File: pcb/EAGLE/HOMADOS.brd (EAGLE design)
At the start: 128.3 x 67.3 mm, 78 parts, among them P1 39-30-02?, P10 39-30-02?, P11 39-30-02?, P12 39-30-02?, P13 39-30-02?, P14 39-30-02?, P15 39-30-02?, P16 39-30-02?, P17 39-30-02?, P18 39-30-02?, P2 39-30-02?, P3 39-30-02?, P4 39-30-02?, P5 39-30-02?, P6 39-30-02?, P7 39-30-02?, P8 39-30-02?, P9 39-30-02?, Q1 T460, Q10 T460, Q11 T460, Q12 T460, Q13 T460, Q14 T460, Q15 T460, Q16 T460, Q2 T460, Q3 T460, Q4 T460, Q5 T460, Q6 T460, Q7 T460, Q8 T460, Q9 T460, U2 ARDUINO-MEGAPRO-5V

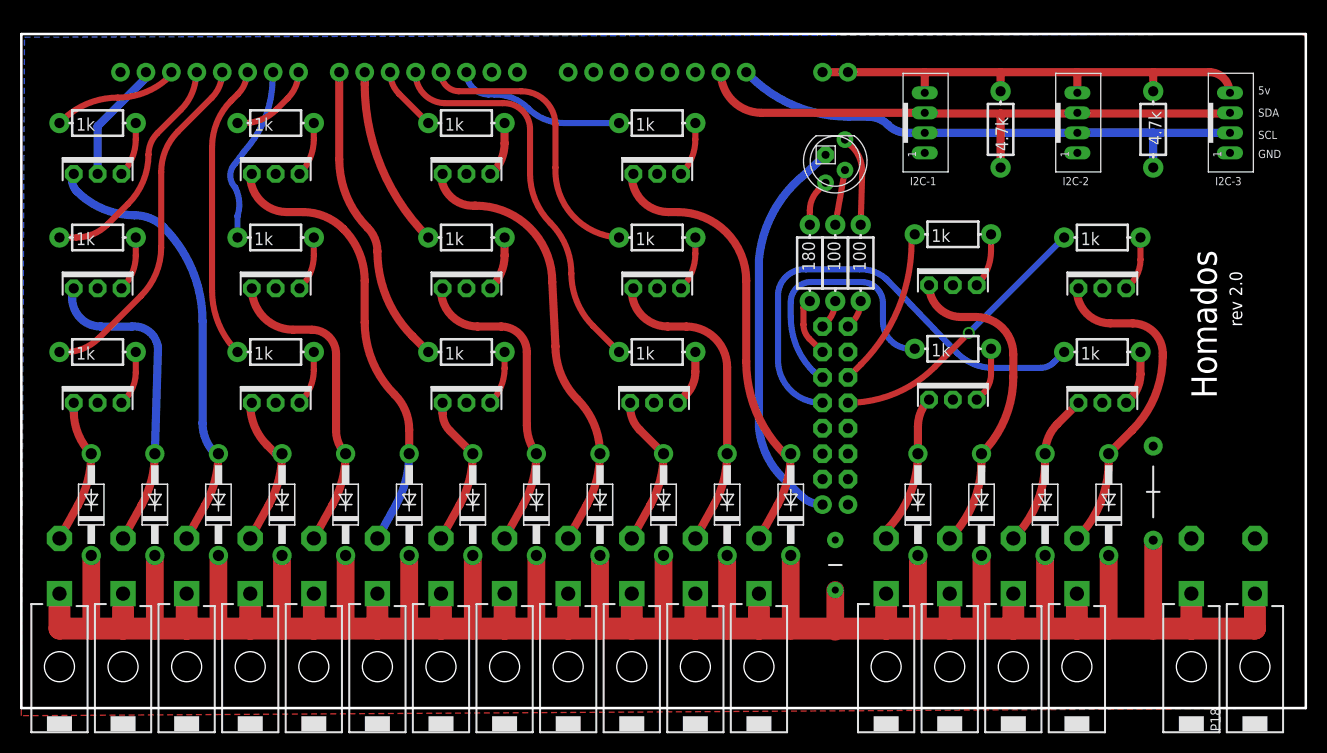
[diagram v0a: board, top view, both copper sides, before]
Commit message: finished revision of homados
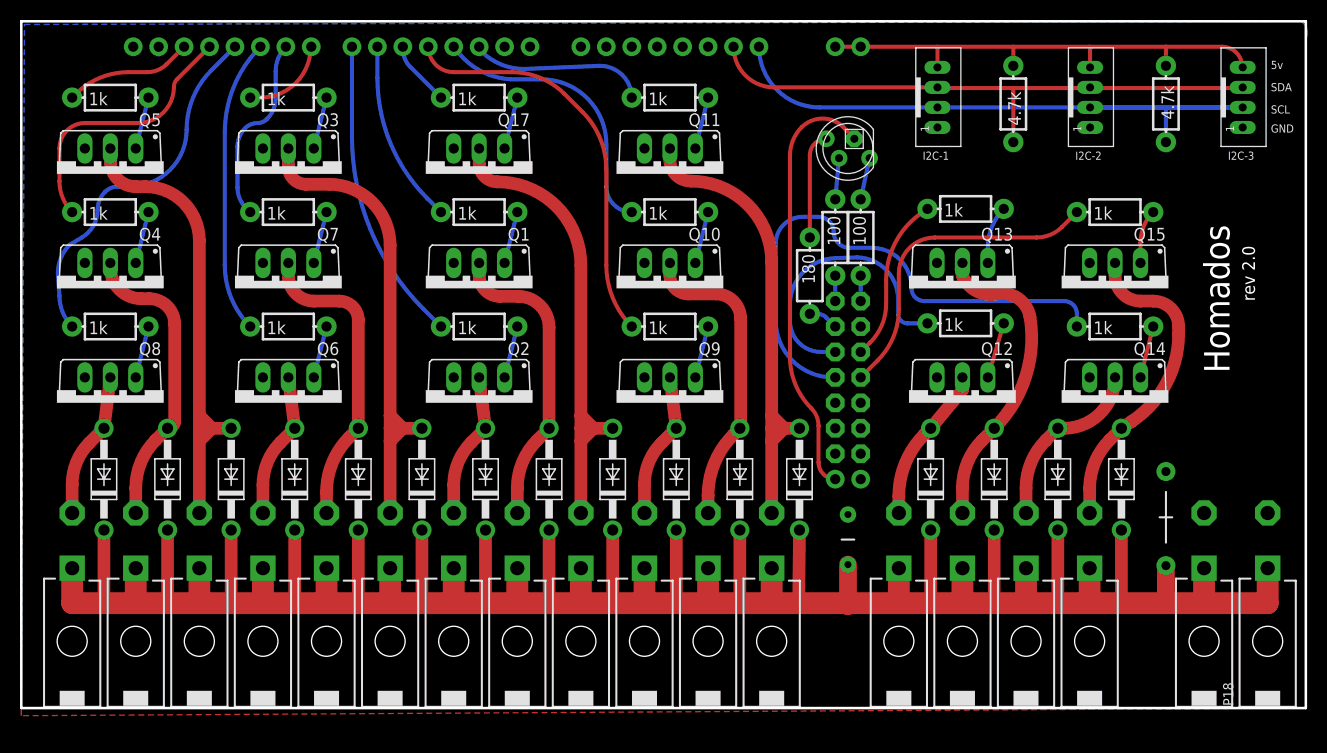
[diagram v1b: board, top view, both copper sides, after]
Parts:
- removed P2: 39-30-02?, con-molex-mini-fit:39-30-?02?
- removed Q16: T460, transistor-npn:TO225AAV
- added P19: 39-30-02?, con-molex-mini-fit:39-30-?02?
- added Q17: (no value), transistor-power:TO220BV
- Q1, Q10, Q11, Q12, Q13, Q14, Q15, Q2, Q3, Q4, Q5, Q6, Q7, Q8, Q9: value T460 -> (none); device transistor-npn:TO225AAV -> transistor-power:TO220BV
- moved Q12 86.4 mm to (94.0, 30.5), turned to 180 degrees
- moved Q6 29.8 mm to (26.7, 30.5), turned to 180 degrees
- moved Q3 29.0 mm to (26.7, 53.3), turned to 180 degrees
- moved Q11 22.9 mm to (64.8, 53.3), turned to 180 degrees
- moved Q9 22.9 mm to (64.8, 30.5), turned to 180 degrees
- moved Q4 20.1 mm to (8.89, 41.9), turned to 180 degrees
- moved Q8 20.1 mm to (8.89, 30.5), turned to 180 degrees
- moved Q14 20.0 mm to (109.2, 30.5), turned to 180 degrees
- moved Q1 11.5 mm to (45.7, 41.9), turned to 180 degrees
- moved Q5 11.5 mm to (8.89, 53.3), turned to 180 degrees
- moved Q15 11.5 mm to (109.2, 41.9), turned to 180 degrees
- moved Q2 11.5 mm to (45.7, 30.5), turned to 180 degrees
- moved Q7 11.5 mm to (26.7, 41.9), turned to 180 degrees
- moved Q13 11.2 mm to (94.0, 41.9), turned to 180 degrees
- moved P13 2.84 mm to (74.9, 14.0)
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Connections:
- removed net N$39: D10.A, P11.2, Q11.1
- removed net N$43: D11.A, P12.2, Q10.1
- removed net N$47: D12.A, P13.2, Q9.1
- removed net N$51: D13.A, P14.2, Q16.1
- removed net N$55: D14.A, P15.2, Q15.1
- removed net N$59: D15.A, P16.2, Q14.1
- removed net N$63: D16.A, P17.2, Q13.1
- new net N$16: D3.A, P4.2, Q2.D
- new net N$20: D6.A, P7.2, Q6.D
- new net N$21: D7.A, P8.2, Q5.D
- new net N$24: D14.A, P15.2, Q14.D
- new net N$25: D15.A, P16.2, Q13.D
- new net N$33: D10.A, P11.2, Q9.D
- new net N$5: D12.A, P13.2, Q11.D
- net GND: now also P19.2, Q1.S, Q10.S, Q11.S, Q12.S, Q13.S, Q14.S, Q15.S, Q17.S, Q2.S, Q3.S, Q4.S, Q5.S, Q6.S, Q7.S, Q8.S, Q9.S; no longer P2.2, Q1.2, Q10.2, Q11.2, Q12.2, Q13.2, Q14.2, Q15.2, Q16.2, Q2.2, Q3.2, Q4.2, Q5.2, Q6.2, Q7.2, Q8.2, Q9.2
- net N$10: now also Q1.G; no longer Q2.3
- net N$11: now also D13.A, P14.2, Q15.D; no longer D3.A, P4.2, Q3.1
- net N$14: now also Q2.G; no longer Q3.3
- net N$15: now also D1.A, P1.2, Q1.D; no longer D4.A, P5.2, Q4.1
- net N$18: now also Q3.G; no longer Q4.3
- net N$19: now also D4.A, P5.2, Q3.D; no longer D5.A, P6.2, Q8.1
- net N$2: now also Q17.D; no longer Q1.1
- net N$22: now also Q7.G; no longer Q8.3
- net N$23: now also D11.A, P12.2, Q10.D; no longer D6.A, P7.2, Q7.1
- net N$26: now also Q6.G; no longer Q7.3
- net N$27: now also D8.A, P9.2, Q4.D; no longer D7.A, P8.2, Q6.1
- net N$30: now also Q5.G; no longer Q6.3
- net N$31: now also D16.A, P17.2, Q12.D; no longer D8.A, P9.2, Q5.1
- net N$34: now also Q4.G; no longer Q5.3
- net N$35: now also Q8.D; no longer Q12.1
- net N$38: now also Q8.G; no longer Q12.3
- net N$4: now also D5.A, P6.2, Q7.D; no longer D1.A, P1.2, Q2.1
- net N$42: now also Q9.G; no longer Q11.3
- net N$46: now also Q10.G; no longer Q10.3
- net N$50: now also Q11.G; no longer Q9.3
- net N$54: now also Q15.G; no longer Q16.3
- net N$58: now also Q14.G; no longer Q15.3
- net N$6: now also Q17.G; no longer Q1.3
- net N$62: now also Q13.G; no longer Q14.3
- net N$66: now also Q12.G; no longer Q13.3
- net PWR: now also P19.1; no longer P2.1
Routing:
- net N$21: track 0.00 -> 47.4 mm
- net N$5: track 0.00 -> 47.0 mm
- net N$47: track 43.8 -> 0.00 mm
- net N$51: track 32.9 -> 0.00 mm
- net N$59: track 31.7 -> 0.00 mm
- net N$43: track 30.7 -> 0.00 mm
- net N$25: track 0.00 -> 30.2 mm
- net N$19: track 30.4 -> 48.7 mm
- net N$24: track 0.00 -> 17.2 mm
- net SCL: track 60.7 -> 77.2 mm
- net N$31: track 31.2 -> 15.5 mm
- net N$11: track 15.3 -> 31.0 mm
- net N$39: track 15.4 -> 0.00 mm
- net N$55: track 15.3 -> 0.00 mm
- net N$27: track 44.3 -> 29.3 mm
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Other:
- board size 128.3 x 67.3 mm -> 128.3 x 68.6 mm
